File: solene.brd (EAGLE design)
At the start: 100 x 80 mm, 1 part, among them J1X CLONOLU

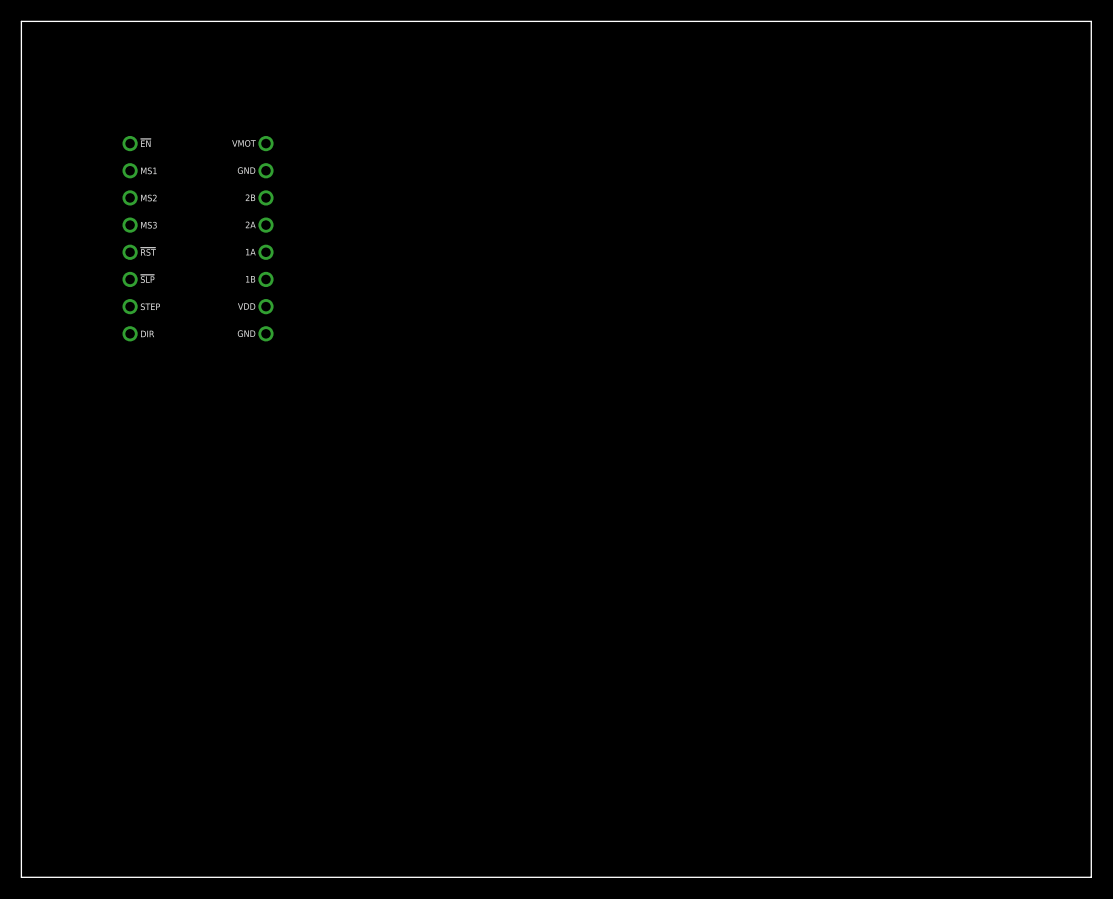
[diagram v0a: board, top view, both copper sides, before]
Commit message: rev 1
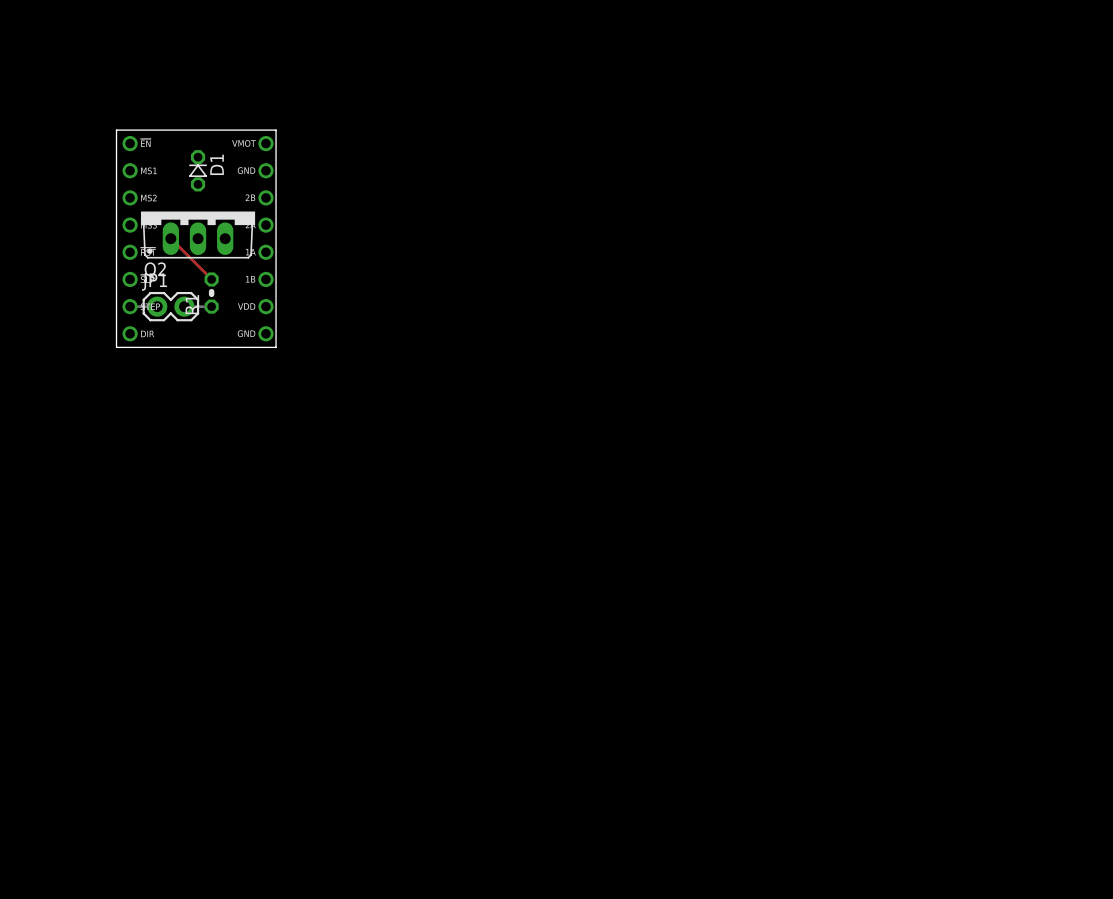
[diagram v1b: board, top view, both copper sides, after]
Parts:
- added D1: 1N4004, diode:D-2.5
- added JP1: (no value), SparkFun-Passives:1X02
- added Q2: IRF540, transistor-power:TO220BV
- added R1: 2k2, rcl:0204V
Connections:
- removed net VMOT: J1X.VMOT
- new net N$1: J1X.STEP, JP1.1
- new net N$2: JP1.2, R1.1
- new net N$3: Q2.G, R1.2
- new net N$4: D1.C, J1X.2B, J1X.VMOT
- new net N$5: D1.A, J1X.2A, Q2.D
- net GND: now also Q2.S
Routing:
- net N$3: track 0.00 -> 5.39 mm
- net N$2: track 0.00 -> 2.54 mm
- net N$1: track 0.00 -> 2.54 mm
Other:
- board size 100 x 80 mm -> 14.9 x 20.3 mm
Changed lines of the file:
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@@
 <layer number="97" name="Info" color="7" fill="1" visible="no" active="no"/>
 <layer number="98" name="Guide" color="6" fill="1" visible="no" active="no"/>
+<layer number="99" name="SpiceOrder" color="5" fill="1" visible="no" active="no"/>
 <layer number="100" name="Muster" color="7" fill="1" visible="no" active="no"/>
 <layer number="101" name="Patch_Top" color="12" fill="4" visible="no" active="yes"/>
@@
 <layer number="106" name="bPlate" color="7" fill="1" visible="no" active="yes"/>
 <layer number="107" name="Crop" color="7" fill="1" visible="no" active="yes"/>
+<layer number="108" name="tplace-old" color="10" fill="1" visible="no" active="yes"/>
+<layer number="109" name="ref-old" color="11" fill="1" visible="no" active="yes"/>
 <layer number="116" name="Patch_BOT" color="9" fill="4" visible="no" active="yes"/>
 <layer number="121" name="_tsilk" color="7" fill="1" visible="no" active="yes"/>
 <layer number="122" name="_bsilk" color="7" fill="1" visible="no" active="yes"/>
+<layer number="125" name="_tNames" color="7" fill="1" visible="no" active="yes"/>
+<layer number="144" name="Drill_legend" color="7" fill="1" visible="no" active="yes"/>
 <layer number="151" name="HeatSink" color="7" fill="1" visible="no" active="yes"/>
+<layer number="199" name="Contour" color="7" fill="1" visible="no" active="yes"/>
 <layer number="200" name="200bmp" color="1" fill="10" visible="no" active="yes"/>
 <layer number="201" name="201bmp" color="2" fill="10" visible="no" active="yes"/>
@@
 <layer number="207" name="207bmp" color="8" fill="10" visible="no" active="yes"/>
 <layer number="208" name="208bmp" color="9" fill="10" visible="no" active="yes"/>
+<layer number="209" name="209bmp" color="7" fill="1" visible="no" active="yes"/>
+<layer number="210" name="210bmp" color="7" fill="1" visible="no" active="yes"/>
+<layer number="211" name="211bmp" color="7" fill="1" visible="no" active="yes"/>
+<layer number="212" name="212bmp" color="7" fill="1" visible="no" active="yes"/>
+<layer number="213" name="213bmp" color="7" fill="1" visible="no" active="yes"/>
+<layer number="214" name="214bmp" color="7" fill="1" visible="no" active="yes"/>
+<layer number="215" name="215bmp" color="7" fill="1" visible="no" active="yes"/>
+<layer number="216" name="216bmp" color="7" fill="1" visible="no" active="yes"/>
+<layer number="217" name="217bmp" color="18" fill="1" visible="no" active="no"/>
+<layer number="218" name="218bmp" color="19" fill="1" visible="no" active="no"/>
+<layer number="219" name="219bmp" color="20" fill="1" visible="no" active="no"/>
+<layer number="220" name="220bmp" color="21" fill="1" visible="no" active="no"/>
+<layer number="221" name="221bmp" color="22" fill="1" visible="no" active="no"/>
+<layer number="222" name="222bmp" color="23" fill="1" visible="no" active="no"/>
+<layer number="223" name="223bmp" color="24" fill="1" visible="no" active="no"/>
+<layer number="224" name="224bmp" color="25" fill="1" visible="no" active="no"/>
 <layer number="250" name="Descript" color="3" fill="1" visible="no" active="no"/>
 <layer number="251" name="SMDround" color="12" fill="11" visible="no" active="no"/>
@@
 <board>
 <plain>
-<wire x1="0" y1="0" x2="100" y2="0" width="0" layer="20"/>
-<wire x1="100" y1="0" x2="100" y2="80" width="0" layer="20"/>
-<wire x1="100" y1="80" x2="0" y2="80" width="0" layer="20"/>
-<wire x1="0" y1="80" x2="0" y2="0" width="0" layer="20"/>
+<wire x1="8.89" y1="49.53" x2="23.8" y2="49.53" width="0" layer="20"/>
+<wire x1="23.8" y1="49.53" x2="23.8" y2="69.84" width="0" layer="20"/>
+<wire x1="23.8" y1="69.84" x2="8.89" y2="69.84" width="0" layer="20"/>
+<wire x1="8.89" y1="69.84" x2="8.89" y2="49.53" width="0" layer="20"/>
 </plain>
 <attributes>
@@
 <elements>
 <element name="J1X" library="pololu-allegro" package="CLONOLU" value="CLONOLU" x="16.51" y="59.69"/>
+<element name="JP1" library="SparkFun-Passives" package="1X02" value="" x="12.7" y="53.34"/>
+<element name="Q2" library="transistor-power" package="TO220BV" value="IRF540" x="16.51" y="62.23"/>
+<element name="D1" library="diode" package="D-2.5" value="1N4004" x="16.51" y="66.04" rot="R270"/>
+<element name="R1" library="rcl" package="0204V" value="2k2" x="17.78" y="54.61" rot="R90"/>
 </elements>
 <signals>
-<signal name="VMOT">
-<contactref element="J1X" pad="VMOT"/>
-</signal>
 <signal name="VDD">
 <contactref element="J1X" pad="VDD"/>
@@
 <contactref element="J1X" pad="GND$2"/>
 <contactref element="J1X" pad="GND$1"/>
-<wire x1="22.86" y1="66.04" x2="22.86" y2="50.8" width="0" layer="19" extent="1-1"/>
+<contactref element="Q2" pad="S"/>
+<wire x1="19.05" y1="59.69" x2="22.86" y2="66.04" width="0" layer="19" extent="1-1"/>
+<wire x1="22.86" y1="50.8" x2="19.05" y2="59.69" width="0" layer="19" extent="1-1"/>
+</signal>
+<signal name="N$1">
+<contactref element="JP1" pad="1"/>
+<contactref element="J1X" pad="STEP"/>
+<wire x1="12.7" y1="53.34" x2="10.16" y2="53.34" width="0.254" layer="16"/>
+</signal>
+<signal name="N$3">
+<contactref element="Q2" pad="G"/>
+<contactref element="R1" pad="2"/>
+<wire x1="13.97" y1="59.69" x2="17.78" y2="55.88" width="0.254" layer="1"/>
+</signal>
+<signal name="N$2">
+<contactref element="JP1" pad="2"/>
+<contactref element="R1" pad="1"/>
+<wire x1="15.24" y1="53.34" x2="17.78" y2="53.34" width="0.254" layer="16"/>
+</signal>
+<signal name="N$4">
+<contactref element="J1X" pad="VMOT"/>
+<contactref element="J1X" pad="2B"/>
+<contactref element="D1" pad="C"/>
+<wire x1="22.86" y1="63.5" x2="22.86" y2="68.58" width="0" layer="19" extent="1-1"/>
+<wire x1="16.51" y1="67.31" x2="22.86" y2="68.58" width="0" layer="19" extent="1-1"/>
+</signal>
+<signal name="N$5">
+<contactref element="J1X" pad="2A"/>
+<contactref element="D1" pad="A"/>
+<contactref element="Q2" pad="D"/>
+<wire x1="16.51" y1="59.69" x2="16.51" y2="64.77" width="0" layer="19" extent="1-16"/>
+<wire x1="16.51" y1="59.69" x2="22.86" y2="60.96" width="0" layer="19" extent="1-1"/>
 </signal>
 </signals>

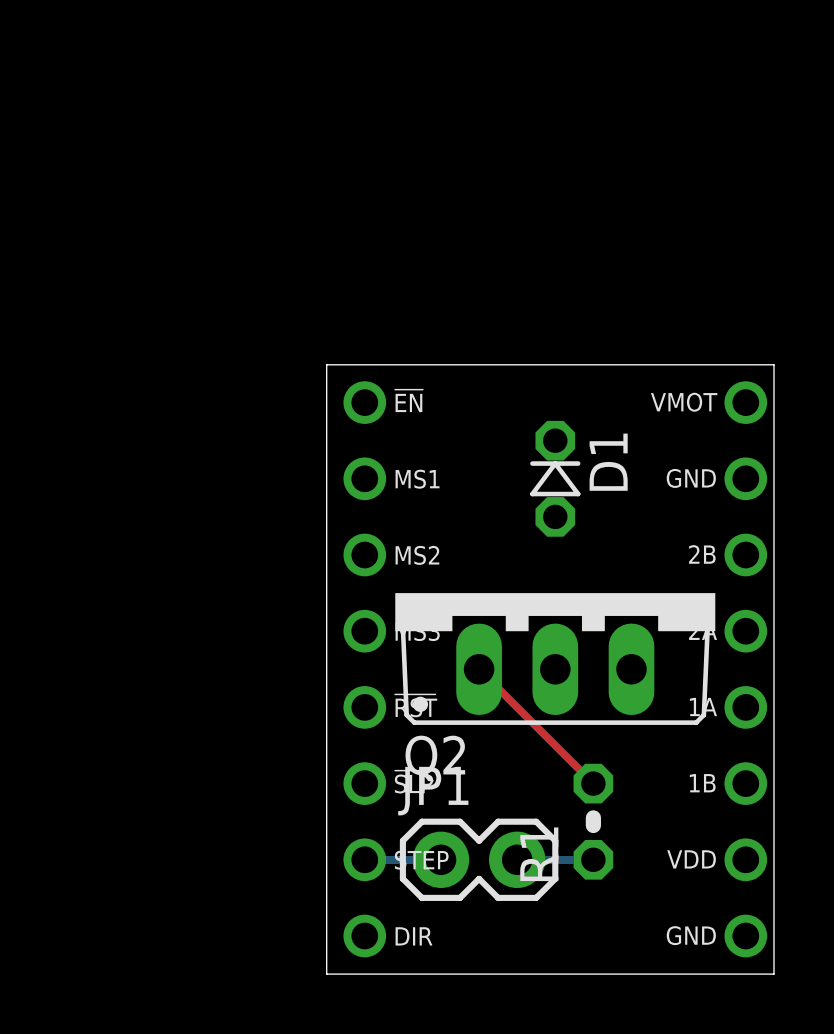
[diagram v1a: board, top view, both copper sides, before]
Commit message: rev 1a
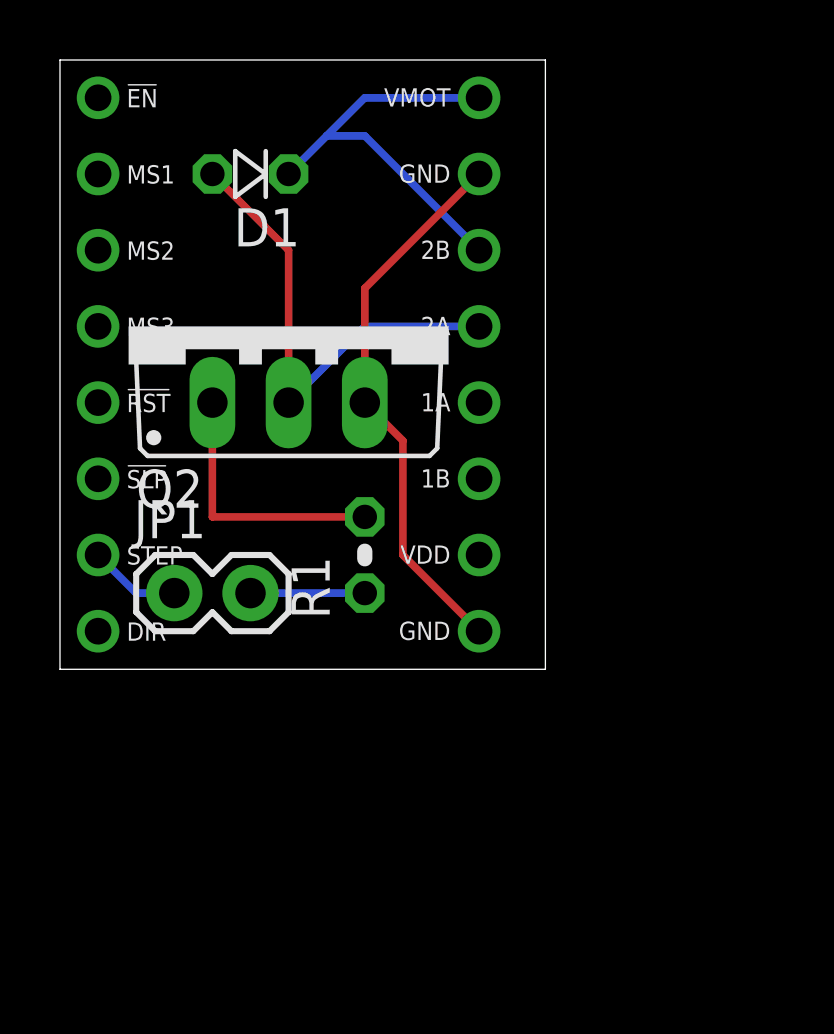
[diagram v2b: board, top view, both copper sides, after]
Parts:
- moved D1 14.4 mm to (6.35, 76.2), turned to 180 degrees
- moved J1X 13.5 mm to (7.62, 69.8)
- moved Q2 12.6 mm to (7.62, 71.1)
- moved JP1 12.6 mm to (3.81, 62.2)
- moved R1 11.7 mm to (10.2, 63.5)
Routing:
- net GND: track 0.00 -> 18.4 mm
- net N$5: track 0.00 -> 16.1 mm
- net N$4: track 0.00 -> 14.1 mm
- net N$3: track 5.39 -> 8.89 mm
- net N$2: track 2.54 -> 3.81 mm
- net N$1: track 2.54 -> 3.07 mm
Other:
- board size 14.9 x 20.3 mm -> 16.2 x 20.3 mm
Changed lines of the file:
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@@
 <drawing>
 <settings>
-<setting alwaysvectorfont="yes"/>
+<setting alwaysvectorfont="no"/>
 <setting verticaltext="up"/>
 </settings>
@@
 <board>
 <plain>
-<wire x1="8.89" y1="49.53" x2="23.8" y2="49.53" width="0" layer="20"/>
-<wire x1="23.8" y1="49.53" x2="23.8" y2="69.84" width="0" layer="20"/>
-<wire x1="23.8" y1="69.84" x2="8.89" y2="69.84" width="0" layer="20"/>
-<wire x1="8.89" y1="69.84" x2="8.89" y2="49.53" width="0" layer="20"/>
+<wire x1="0" y1="59.69" x2="16.18" y2="59.69" width="0" layer="20"/>
+<wire x1="16.18" y1="59.69" x2="16.18" y2="80" width="0" layer="20"/>
+<wire x1="16.18" y1="80" x2="0" y2="80" width="0" layer="20"/>
+<wire x1="0" y1="80" x2="0" y2="59.69" width="0" layer="20"/>
 </plain>
 <attributes>
@@
 </autorouter>
 <elements>
-<element name="J1X" library="pololu-allegro" package="CLONOLU" value="CLONOLU" x="16.51" y="59.69"/>
-<element name="JP1" library="SparkFun-Passives" package="1X02" value="" x="12.7" y="53.34"/>
-<element name="Q2" library="transistor-power" package="TO220BV" value="IRF540" x="16.51" y="62.23"/>
-<element name="D1" library="diode" package="D-2.5" value="1N4004" x="16.51" y="66.04" rot="R270"/>
-<element name="R1" library="rcl" package="0204V" value="2k2" x="17.78" y="54.61" rot="R90"/>
+<element name="J1X" library="pololu-allegro" package="CLONOLU" value="CLONOLU" x="7.62" y="69.85"/>
+<element name="JP1" library="SparkFun-Passives" package="1X02" value="" x="3.81" y="62.23"/>
+<element name="Q2" library="transistor-power" package="TO220BV" value="IRF540" x="7.62" y="71.12"/>
+<element name="D1" library="diode" package="D-2.5" value="1N4004" x="6.35" y="76.2" rot="R180"/>
+<element name="R1" library="rcl" package="0204V" value="2k2" x="10.16" y="63.5" rot="R90"/>
 </elements>
 <signals>
@@
 <contactref element="J1X" pad="GND$1"/>
 <contactref element="Q2" pad="S"/>
-<wire x1="19.05" y1="59.69" x2="22.86" y2="66.04" width="0" layer="19" extent="1-1"/>
-<wire x1="22.86" y1="50.8" x2="19.05" y2="59.69" width="0" layer="19" extent="1-1"/>
+<wire x1="11.43" y1="63.5" x2="13.97" y2="60.96" width="0.254" layer="1"/>
+<wire x1="11.43" y1="67.31" x2="11.43" y2="63.5" width="0.254" layer="1"/>
+<wire x1="10.16" y1="68.58" x2="11.43" y2="67.31" width="0.254" layer="1"/>
+<wire x1="10.16" y1="72.39" x2="13.97" y2="76.2" width="0.254" layer="1"/>
+<wire x1="10.16" y1="68.58" x2="10.16" y2="72.39" width="0.254" layer="1"/>
 </signal>
 <signal name="N$1">
 <contactref element="JP1" pad="1"/>
 <contactref element="J1X" pad="STEP"/>
-<wire x1="12.7" y1="53.34" x2="10.16" y2="53.34" width="0.254" layer="16"/>
+<wire x1="2.54" y1="62.23" x2="1.27" y2="63.5" width="0.254" layer="16"/>
+<wire x1="3.81" y1="62.23" x2="2.54" y2="62.23" width="0.254" layer="16"/>
 </signal>
 <signal name="N$3">
 <contactref element="Q2" pad="G"/>
 <contactref element="R1" pad="2"/>
-<wire x1="13.97" y1="59.69" x2="17.78" y2="55.88" width="0.254" layer="1"/>
+<wire x1="5.08" y1="64.77" x2="10.16" y2="64.77" width="0.254" layer="1"/>
+<wire x1="5.08" y1="68.58" x2="5.08" y2="64.77" width="0.254" layer="1"/>
 </signal>
 <signal name="N$2">
 <contactref element="JP1" pad="2"/>
 <contactref element="R1" pad="1"/>
-<wire x1="15.24" y1="53.34" x2="17.78" y2="53.34" width="0.254" layer="16"/>
+<wire x1="6.35" y1="62.23" x2="10.16" y2="62.23" width="0.254" layer="16"/>
 </signal>
 <signal name="N$4">
@@
 <contactref element="J1X" pad="2B"/>
 <contactref element="D1" pad="C"/>
-<wire x1="22.86" y1="63.5" x2="22.86" y2="68.58" width="0" layer="19" extent="1-1"/>
-<wire x1="16.51" y1="67.31" x2="22.86" y2="68.58" width="0" layer="19" extent="1-1"/>
+<wire x1="10.16" y1="78.74" x2="8.89" y2="77.47" width="0.254" layer="16"/>
+<wire x1="8.89" y1="77.47" x2="7.62" y2="76.2" width="0.254" layer="16"/>
+<wire x1="13.97" y1="78.74" x2="10.16" y2="78.74" width="0.254" layer="16"/>
+<wire x1="10.16" y1="77.47" x2="13.97" y2="73.66" width="0.254" layer="16"/>
+<wire x1="8.89" y1="77.47" x2="10.16" y2="77.47" width="0.254" layer="16"/>
 </signal>
 <signal name="N$5">
@@
 <contactref element="D1" pad="A"/>
 <contactref element="Q2" pad="D"/>
-<wire x1="16.51" y1="59.69" x2="16.51" y2="64.77" width="0" layer="19" extent="1-16"/>
-<wire x1="16.51" y1="59.69" x2="22.86" y2="60.96" width="0" layer="19" extent="1-1"/>
+<wire x1="7.62" y1="73.66" x2="5.08" y2="76.2" width="0.254" layer="1"/>
+<wire x1="7.62" y1="68.58" x2="7.62" y2="73.66" width="0.254" layer="1"/>
+<wire x1="10.16" y1="71.12" x2="13.97" y2="71.12" width="0.254" layer="16"/>
+<wire x1="7.62" y1="68.58" x2="10.16" y2="71.12" width="0.254" layer="16"/>
 </signal>
 </signals>
